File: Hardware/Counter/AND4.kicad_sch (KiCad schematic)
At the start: 10 parts, among them Q21 FDN360P, Q22 FDN360P, Q23 FDN360P, Q24 FDN335N, Q25 FDN335N, Q26 FDN335N, Q27 FDN335N, Q28 FDN335N, U8 FDN360P, U9 FDN360P

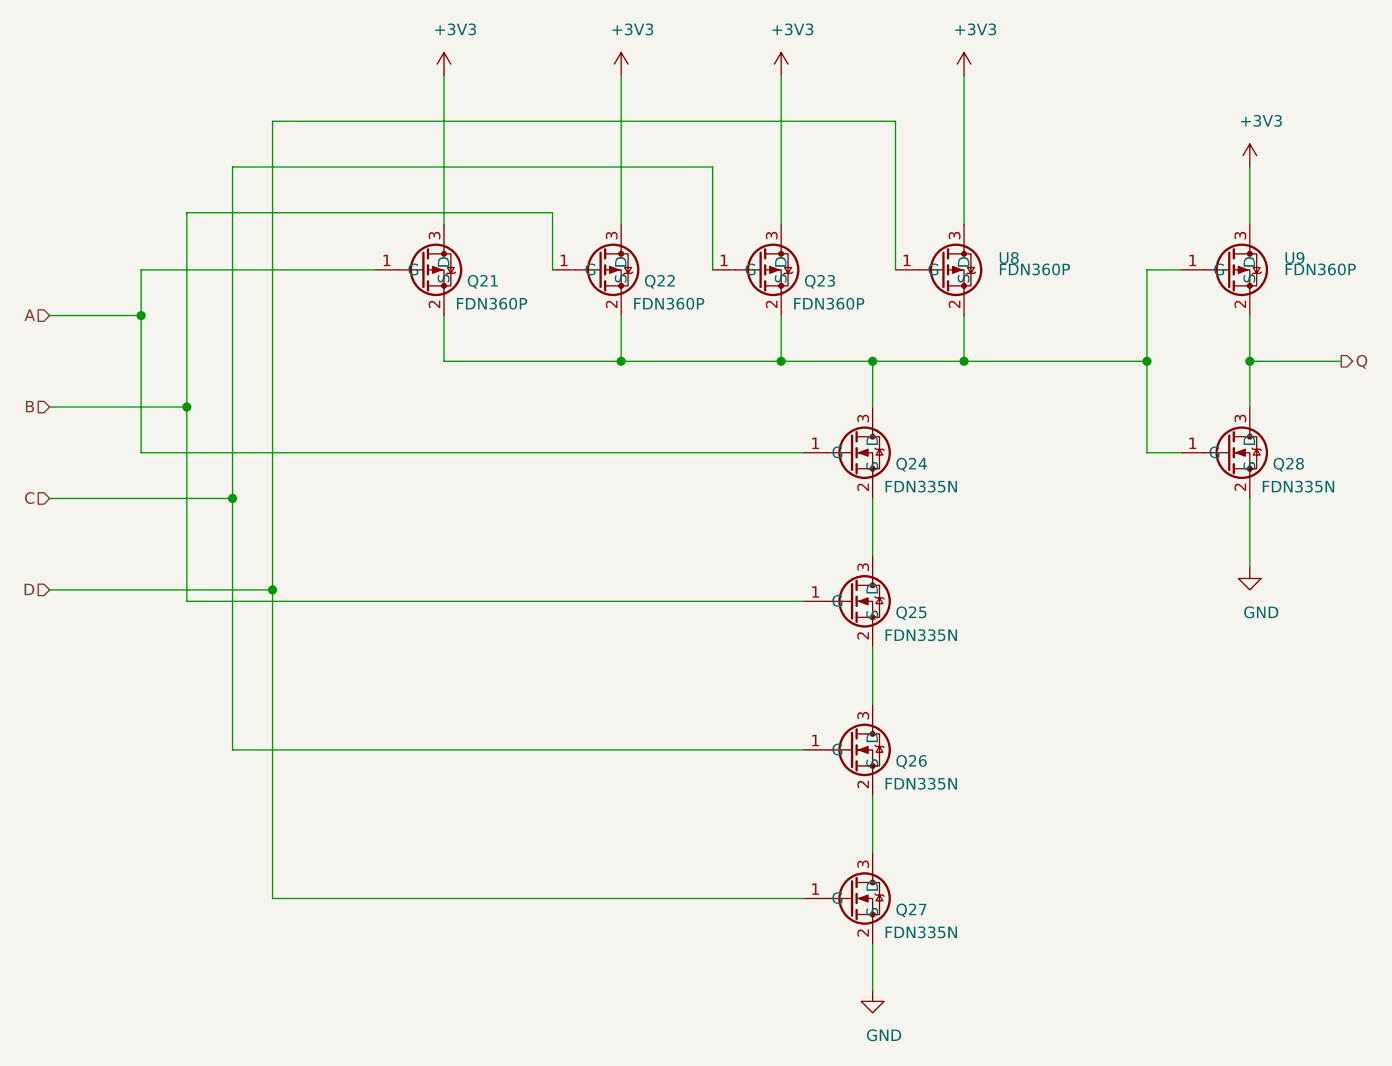
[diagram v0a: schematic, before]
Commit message: working on connectin bits together
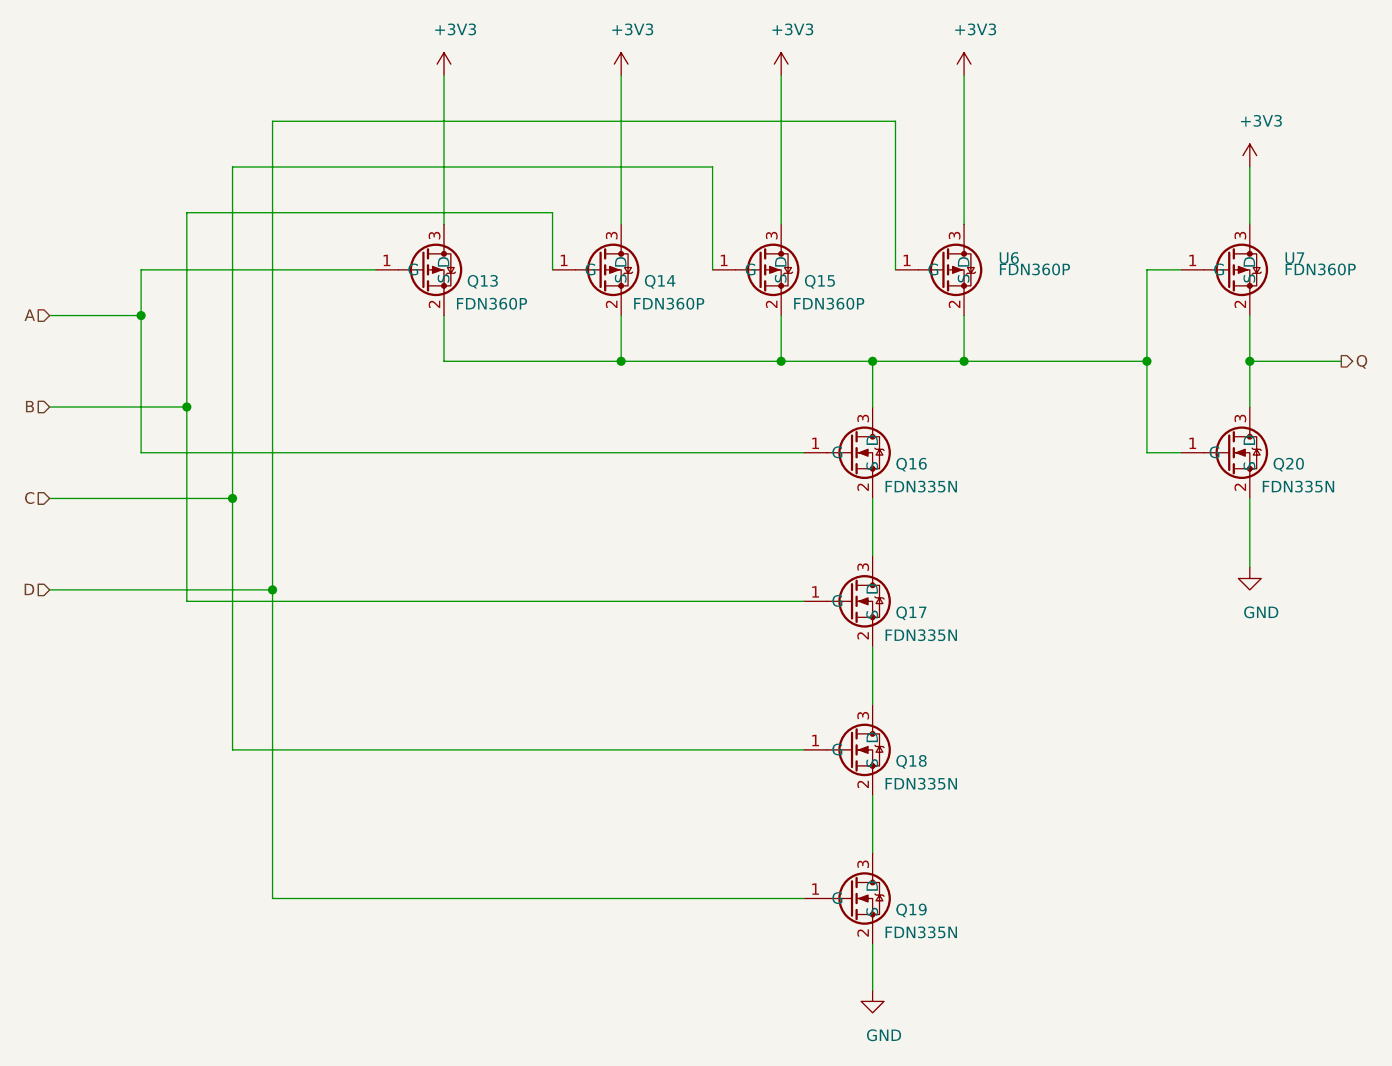
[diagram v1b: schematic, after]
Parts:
- renumbered Q21 to Q13, Q22 to Q14, Q23 to Q15, Q24 to Q16, Q25 to Q17, Q26 to Q18, Q27 to Q19, Q28 to Q20, U8 to U6, U9 to U7
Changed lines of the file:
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@@
   (symbol (lib_id "power:+3V3") (at 96.52 54.61 0)
     (in_bom yes) (on_board yes)
-    (property "Reference" "#PWR0139" (id 0) (at 96.52 58.42 0)
+    (property "Reference" "#PWR0132" (id 0) (at 96.52 58.42 0)
       (effects (font (size 1.27 1.27)) hide)
     )
@@
   (symbol (lib_id "power:+3V3") (at 116.205 54.61 0)
     (in_bom yes) (on_board yes)
-    (property "Reference" "#PWR0137" (id 0) (at 116.205 58.42 0)
+    (property "Reference" "#PWR0130" (id 0) (at 116.205 58.42 0)
       (effects (font (size 1.27 1.27)) hide)
     )
@@
   (symbol (lib_id "power:+3V3") (at 133.985 54.61 0)
     (in_bom yes) (on_board yes)
-    (property "Reference" "#PWR0138" (id 0) (at 133.985 58.42 0)
+    (property "Reference" "#PWR0131" (id 0) (at 133.985 58.42 0)
       (effects (font (size 1.27 1.27)) hide)
     )
@@
   (symbol (lib_id "power:+3V3") (at 154.305 54.61 0)
     (in_bom yes) (on_board yes)
-    (property "Reference" "#PWR0140" (id 0) (at 154.305 58.42 0)
+    (property "Reference" "#PWR0133" (id 0) (at 154.305 58.42 0)
       (effects (font (size 1.27 1.27)) hide)
     )
@@
   (symbol (lib_id "power:+3V3") (at 186.055 64.77 0)
     (in_bom yes) (on_board yes)
-    (property "Reference" "#PWR0143" (id 0) (at 186.055 68.58 0)
+    (property "Reference" "#PWR0136" (id 0) (at 186.055 68.58 0)
       (effects (font (size 1.27 1.27)) hide)
     )
@@
   (symbol (lib_id "power:GND") (at 144.145 156.21 0)
     (in_bom yes) (on_board yes)
-    (property "Reference" "#PWR0141" (id 0) (at 144.145 162.56 0)
+    (property "Reference" "#PWR0134" (id 0) (at 144.145 162.56 0)
       (effects (font (size 1.27 1.27)) hide)
     )
@@
   (symbol (lib_id "power:GND") (at 186.055 109.22 0)
     (in_bom yes) (on_board yes)
-    (property "Reference" "#PWR0142" (id 0) (at 186.055 115.57 0)
+    (property "Reference" "#PWR0135" (id 0) (at 186.055 115.57 0)
       (effects (font (size 1.27 1.27)) hide)
     )
@@
   (symbol (lib_name "Custom_Transistors:FDN360P_1") (lib_id "Custom_Transistors:FDN360P") (at 96.52 76.2 0)
     (in_bom yes) (on_board yes)
-    (property "Reference" "Q21" (id 0) (at 99.06 77.47 0)
+    (property "Reference" "Q13" (id 0) (at 99.06 77.47 0)
       (effects (font (size 1.27 1.27)) (justify left))
     )
@@
   (symbol (lib_name "Custom_Transistors:FDN360P_2") (lib_id "Custom_Transistors:FDN360P") (at 116.205 76.2 0)
     (in_bom yes) (on_board yes)
-    (property "Reference" "Q22" (id 0) (at 118.745 77.47 0)
+    (property "Reference" "Q14" (id 0) (at 118.745 77.47 0)
       (effects (font (size 1.27 1.27)) (justify left))
     )
@@
   (symbol (lib_name "Custom_Transistors:FDN360P_3") (lib_id "Custom_Transistors:FDN360P") (at 133.985 76.2 0)
     (in_bom yes) (on_board yes)
-    (property "Reference" "Q23" (id 0) (at 136.525 77.47 0)
+    (property "Reference" "Q15" (id 0) (at 136.525 77.47 0)
       (effects (font (size 1.27 1.27)) (justify left))
     )
@@
   (symbol (lib_id "Custom_Transistors:FDN335N") (at 144.145 96.52 0)
     (in_bom yes) (on_board yes)
-    (property "Reference" "Q24" (id 0) (at 146.685 97.79 0)
+    (property "Reference" "Q16" (id 0) (at 146.685 97.79 0)
       (effects (font (size 1.27 1.27)) (justify left))
     )
@@
   (symbol (lib_id "Custom_Transistors:FDN335N") (at 144.145 113.03 0)
     (in_bom yes) (on_board yes)
-    (property "Reference" "Q25" (id 0) (at 146.685 114.3 0)
+    (property "Reference" "Q17" (id 0) (at 146.685 114.3 0)
       (effects (font (size 1.27 1.27)) (justify left))
     )
@@
   (symbol (lib_id "Custom_Transistors:FDN335N") (at 144.145 129.54 0)
     (in_bom yes) (on_board yes)
-    (property "Reference" "Q26" (id 0) (at 146.685 130.81 0)
+    (property "Reference" "Q18" (id 0) (at 146.685 130.81 0)
       (effects (font (size 1.27 1.27)) (justify left))
     )
@@
   (symbol (lib_id "Custom_Transistors:FDN335N") (at 144.145 146.05 0)
     (in_bom yes) (on_board yes)
-    (property "Reference" "Q27" (id 0) (at 146.685 147.32 0)
+    (property "Reference" "Q19" (id 0) (at 146.685 147.32 0)
       (effects (font (size 1.27 1.27)) (justify left))
     )
@@
   (symbol (lib_name "Custom_Transistors:FDN360P_4") (lib_id "Custom_Transistors:FDN360P") (at 154.305 76.2 0)
     (in_bom yes) (on_board yes)
-    (property "Reference" "U8" (id 0) (at 158.115 74.93 0)
+    (property "Reference" "U6" (id 0) (at 158.115 74.93 0)
       (effects (font (size 1.27 1.27)) (justify left))
     )
@@
   (symbol (lib_id "Custom_Transistors:FDN360P") (at 186.055 76.2 0)
     (in_bom yes) (on_board yes)
-    (property "Reference" "U9" (id 0) (at 189.865 74.93 0)
+    (property "Reference" "U7" (id 0) (at 189.865 74.93 0)
       (effects (font (size 1.27 1.27)) (justify left))
     )
@@
   (symbol (lib_id "Custom_Transistors:FDN335N") (at 186.055 96.52 0)
     (in_bom yes) (on_board yes)
-    (property "Reference" "Q28" (id 0) (at 188.595 97.79 0)
-      (effects (font (size 1.27 1.27)) (justify left))
-    )
+    (property "Reference" "Q20" (id 0) (at 188.595 97.79 0)
+      (effects (font (size 1.27 1.27)) (justify left))
+    )

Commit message: kicad updates
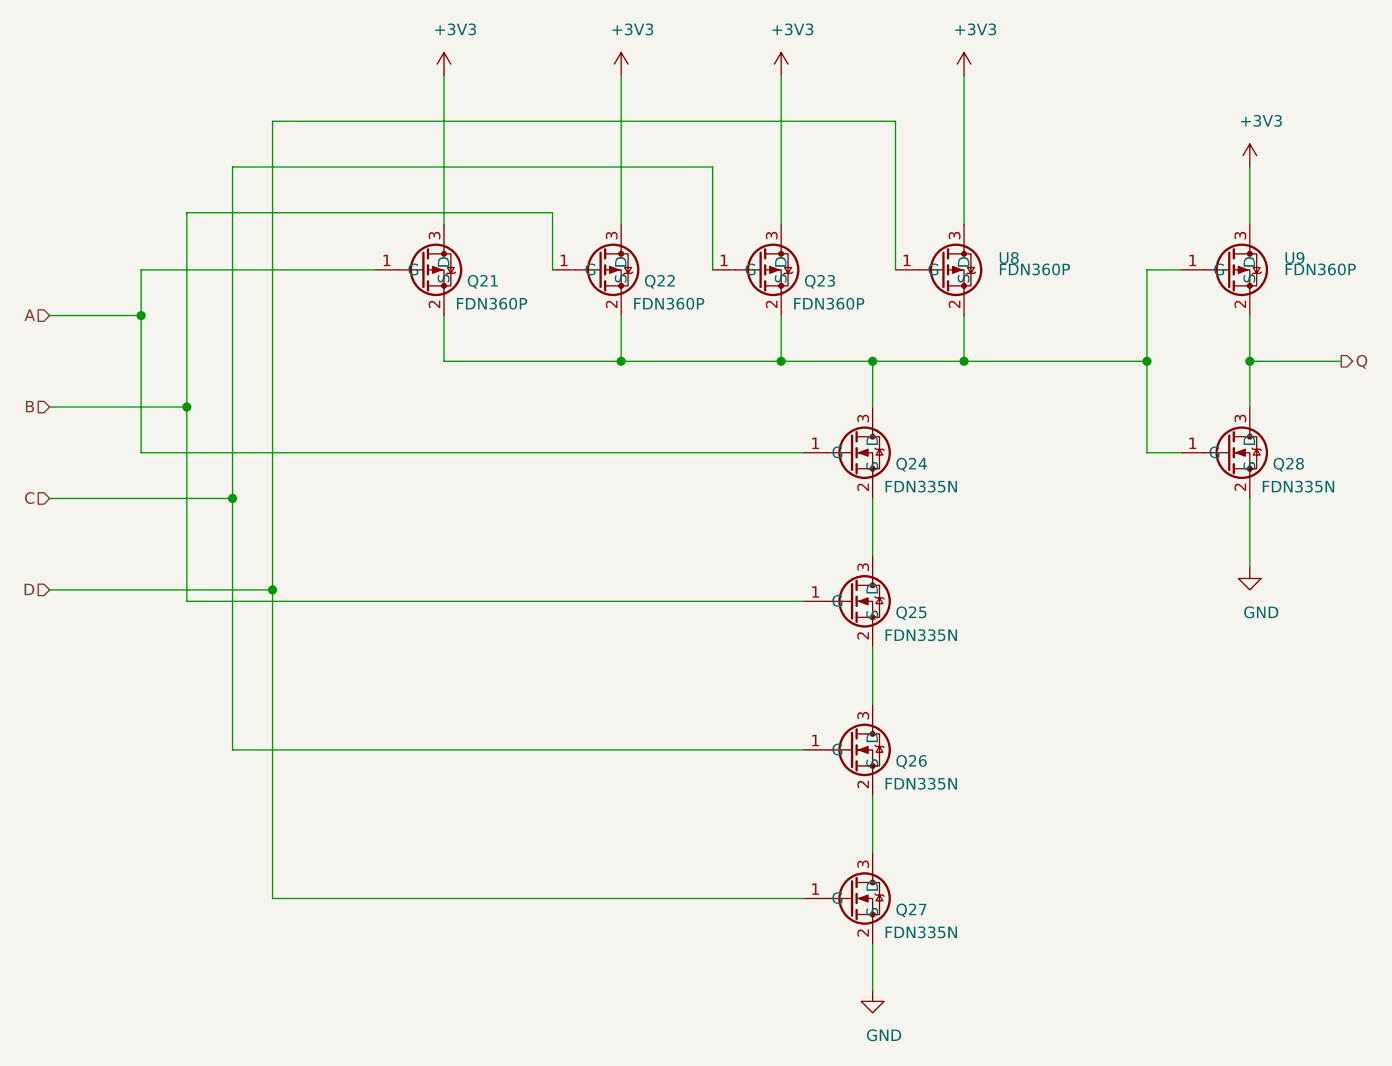
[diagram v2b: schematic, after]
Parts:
- renumbered Q13 to Q21, Q14 to Q22, Q15 to Q23, Q16 to Q24, Q17 to Q25, Q18 to Q26, Q19 to Q27, Q20 to Q28, U6 to U8, U7 to U9
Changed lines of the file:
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@@
   (symbol (lib_id "power:+3V3") (at 96.52 54.61 0)
     (in_bom yes) (on_board yes)
-    (property "Reference" "#PWR0132" (id 0) (at 96.52 58.42 0)
+    (property "Reference" "#PWR0139" (id 0) (at 96.52 58.42 0)
       (effects (font (size 1.27 1.27)) hide)
     )
@@
   (symbol (lib_id "power:+3V3") (at 116.205 54.61 0)
     (in_bom yes) (on_board yes)
-    (property "Reference" "#PWR0130" (id 0) (at 116.205 58.42 0)
+    (property "Reference" "#PWR0137" (id 0) (at 116.205 58.42 0)
       (effects (font (size 1.27 1.27)) hide)
     )
@@
   (symbol (lib_id "power:+3V3") (at 133.985 54.61 0)
     (in_bom yes) (on_board yes)
-    (property "Reference" "#PWR0131" (id 0) (at 133.985 58.42 0)
+    (property "Reference" "#PWR0138" (id 0) (at 133.985 58.42 0)
       (effects (font (size 1.27 1.27)) hide)
     )
@@
   (symbol (lib_id "power:+3V3") (at 154.305 54.61 0)
     (in_bom yes) (on_board yes)
-    (property "Reference" "#PWR0133" (id 0) (at 154.305 58.42 0)
+    (property "Reference" "#PWR0140" (id 0) (at 154.305 58.42 0)
       (effects (font (size 1.27 1.27)) hide)
     )
@@
   (symbol (lib_id "power:+3V3") (at 186.055 64.77 0)
     (in_bom yes) (on_board yes)
-    (property "Reference" "#PWR0136" (id 0) (at 186.055 68.58 0)
+    (property "Reference" "#PWR0143" (id 0) (at 186.055 68.58 0)
       (effects (font (size 1.27 1.27)) hide)
     )
@@
   (symbol (lib_id "power:GND") (at 144.145 156.21 0)
     (in_bom yes) (on_board yes)
-    (property "Reference" "#PWR0134" (id 0) (at 144.145 162.56 0)
+    (property "Reference" "#PWR0141" (id 0) (at 144.145 162.56 0)
       (effects (font (size 1.27 1.27)) hide)
     )
@@
   (symbol (lib_id "power:GND") (at 186.055 109.22 0)
     (in_bom yes) (on_board yes)
-    (property "Reference" "#PWR0135" (id 0) (at 186.055 115.57 0)
+    (property "Reference" "#PWR0142" (id 0) (at 186.055 115.57 0)
       (effects (font (size 1.27 1.27)) hide)
     )
@@
   (symbol (lib_name "Custom_Transistors:FDN360P_1") (lib_id "Custom_Transistors:FDN360P") (at 96.52 76.2 0)
     (in_bom yes) (on_board yes)
-    (property "Reference" "Q13" (id 0) (at 99.06 77.47 0)
+    (property "Reference" "Q21" (id 0) (at 99.06 77.47 0)
       (effects (font (size 1.27 1.27)) (justify left))
     )
@@
   (symbol (lib_name "Custom_Transistors:FDN360P_2") (lib_id "Custom_Transistors:FDN360P") (at 116.205 76.2 0)
     (in_bom yes) (on_board yes)
-    (property "Reference" "Q14" (id 0) (at 118.745 77.47 0)
+    (property "Reference" "Q22" (id 0) (at 118.745 77.47 0)
       (effects (font (size 1.27 1.27)) (justify left))
     )
@@
   (symbol (lib_name "Custom_Transistors:FDN360P_3") (lib_id "Custom_Transistors:FDN360P") (at 133.985 76.2 0)
     (in_bom yes) (on_board yes)
-    (property "Reference" "Q15" (id 0) (at 136.525 77.47 0)
+    (property "Reference" "Q23" (id 0) (at 136.525 77.47 0)
       (effects (font (size 1.27 1.27)) (justify left))
     )
@@
   (symbol (lib_id "Custom_Transistors:FDN335N") (at 144.145 96.52 0)
     (in_bom yes) (on_board yes)
-    (property "Reference" "Q16" (id 0) (at 146.685 97.79 0)
+    (property "Reference" "Q24" (id 0) (at 146.685 97.79 0)
       (effects (font (size 1.27 1.27)) (justify left))
     )
@@
   (symbol (lib_id "Custom_Transistors:FDN335N") (at 144.145 113.03 0)
     (in_bom yes) (on_board yes)
-    (property "Reference" "Q17" (id 0) (at 146.685 114.3 0)
+    (property "Reference" "Q25" (id 0) (at 146.685 114.3 0)
       (effects (font (size 1.27 1.27)) (justify left))
     )
@@
   (symbol (lib_id "Custom_Transistors:FDN335N") (at 144.145 129.54 0)
     (in_bom yes) (on_board yes)
-    (property "Reference" "Q18" (id 0) (at 146.685 130.81 0)
+    (property "Reference" "Q26" (id 0) (at 146.685 130.81 0)
       (effects (font (size 1.27 1.27)) (justify left))
     )
@@
   (symbol (lib_id "Custom_Transistors:FDN335N") (at 144.145 146.05 0)
     (in_bom yes) (on_board yes)
-    (property "Reference" "Q19" (id 0) (at 146.685 147.32 0)
+    (property "Reference" "Q27" (id 0) (at 146.685 147.32 0)
       (effects (font (size 1.27 1.27)) (justify left))
     )
@@
   (symbol (lib_name "Custom_Transistors:FDN360P_4") (lib_id "Custom_Transistors:FDN360P") (at 154.305 76.2 0)
     (in_bom yes) (on_board yes)
-    (property "Reference" "U6" (id 0) (at 158.115 74.93 0)
+    (property "Reference" "U8" (id 0) (at 158.115 74.93 0)
       (effects (font (size 1.27 1.27)) (justify left))
     )
@@
   (symbol (lib_id "Custom_Transistors:FDN360P") (at 186.055 76.2 0)
     (in_bom yes) (on_board yes)
-    (property "Reference" "U7" (id 0) (at 189.865 74.93 0)
+    (property "Reference" "U9" (id 0) (at 189.865 74.93 0)
       (effects (font (size 1.27 1.27)) (justify left))
     )
@@
   (symbol (lib_id "Custom_Transistors:FDN335N") (at 186.055 96.52 0)
     (in_bom yes) (on_board yes)
-    (property "Reference" "Q20" (id 0) (at 188.595 97.79 0)
-      (effects (font (size 1.27 1.27)) (justify left))
-    )
+    (property "Reference" "Q28" (id 0) (at 188.595 97.79 0)
+      (effects (font (size 1.27 1.27)) (justify left))
+    )
